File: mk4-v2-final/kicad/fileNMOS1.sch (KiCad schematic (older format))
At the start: 2 parts, among them Q7 FQB30N06LTM

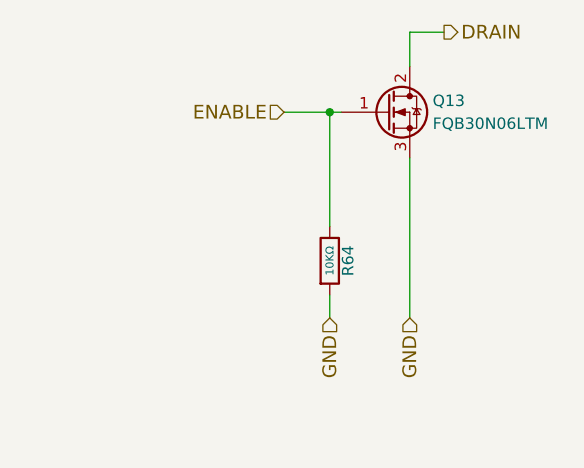
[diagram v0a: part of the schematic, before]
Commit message: all files are in, time to order!
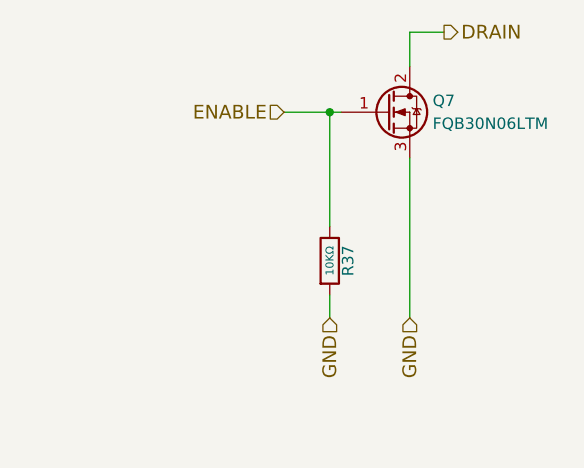
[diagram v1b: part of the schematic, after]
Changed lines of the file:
@@
 AR Path="/59DEA30F/5B17D435/59DF0BE3" Ref="R107"  Part="1"
 AR Path="/59DEA30F/5B17FE95/59DF0BE3" Ref="R109"  Part="1"
-F 0 "R64" V 5230 4900 50  0000 C CNN
+F 0 "R37" V 5230 4900 50  0000 C CNN
 F 1 "10KΩ" V 5150 4900 35  0000 C CNN
 F 2 "Resistors_THT:R_Axial_DIN0204_L3.6mm_D1.6mm_P5.08mm_Horizontal" V 5080 4900 50  0001 C CNN
@@
 AR Path="/59DEA30F/5B17D435/5A2ED2FC" Ref="Q31"  Part="1"
 AR Path="/59DEA30F/5B17FE95/5A2ED2FC" Ref="Q32"  Part="1"
-F 0 "Q13" H 5600 4300 50  0000 L CNN
+F 0 "Q7" H 5600 4300 50  0000 L CNN
 F 1 "FQB30N06LTM" H 5600 4200 50  0000 L CNN
 F 2 "TO_SOT_Packages_SMD:TO-263-3_TabPin2" H 5600 4350 50  0001 C CNN
